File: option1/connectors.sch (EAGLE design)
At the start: 14 parts, among them CON1 PINHEAD_1X06-2, CON2 PINHEAD_1X03-2.54-RA, CON3 CON-4P-JST_GH-RA, CON4 PINHEAD_1X02-2, CON5 PINHEAD_1X02-2, CON8 CON-4P-JST_GH-RA, IC3 TJA1051

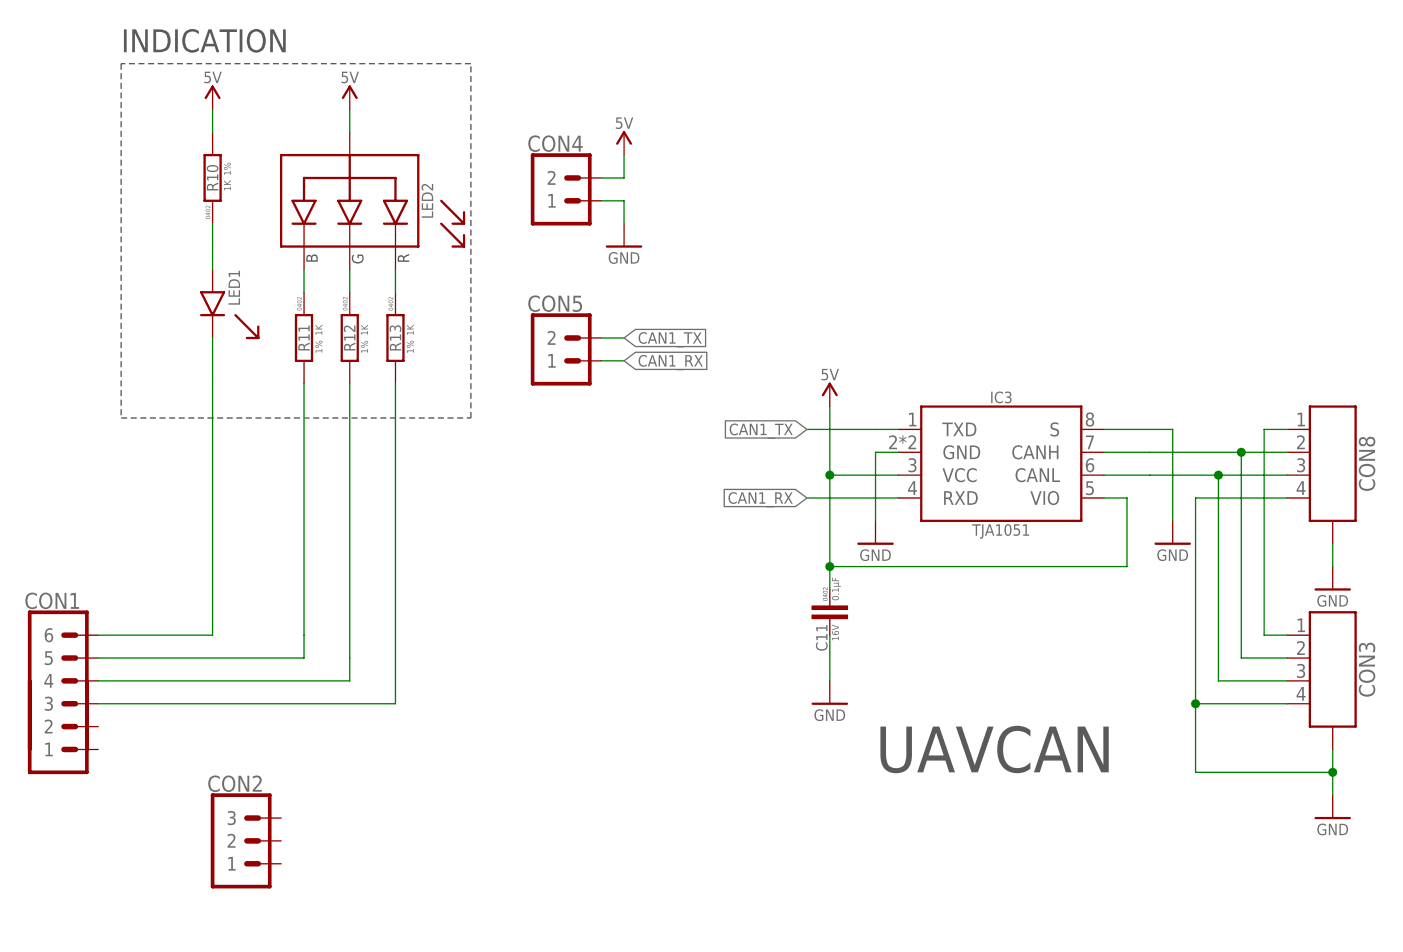
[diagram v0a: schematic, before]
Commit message: Roting is completed
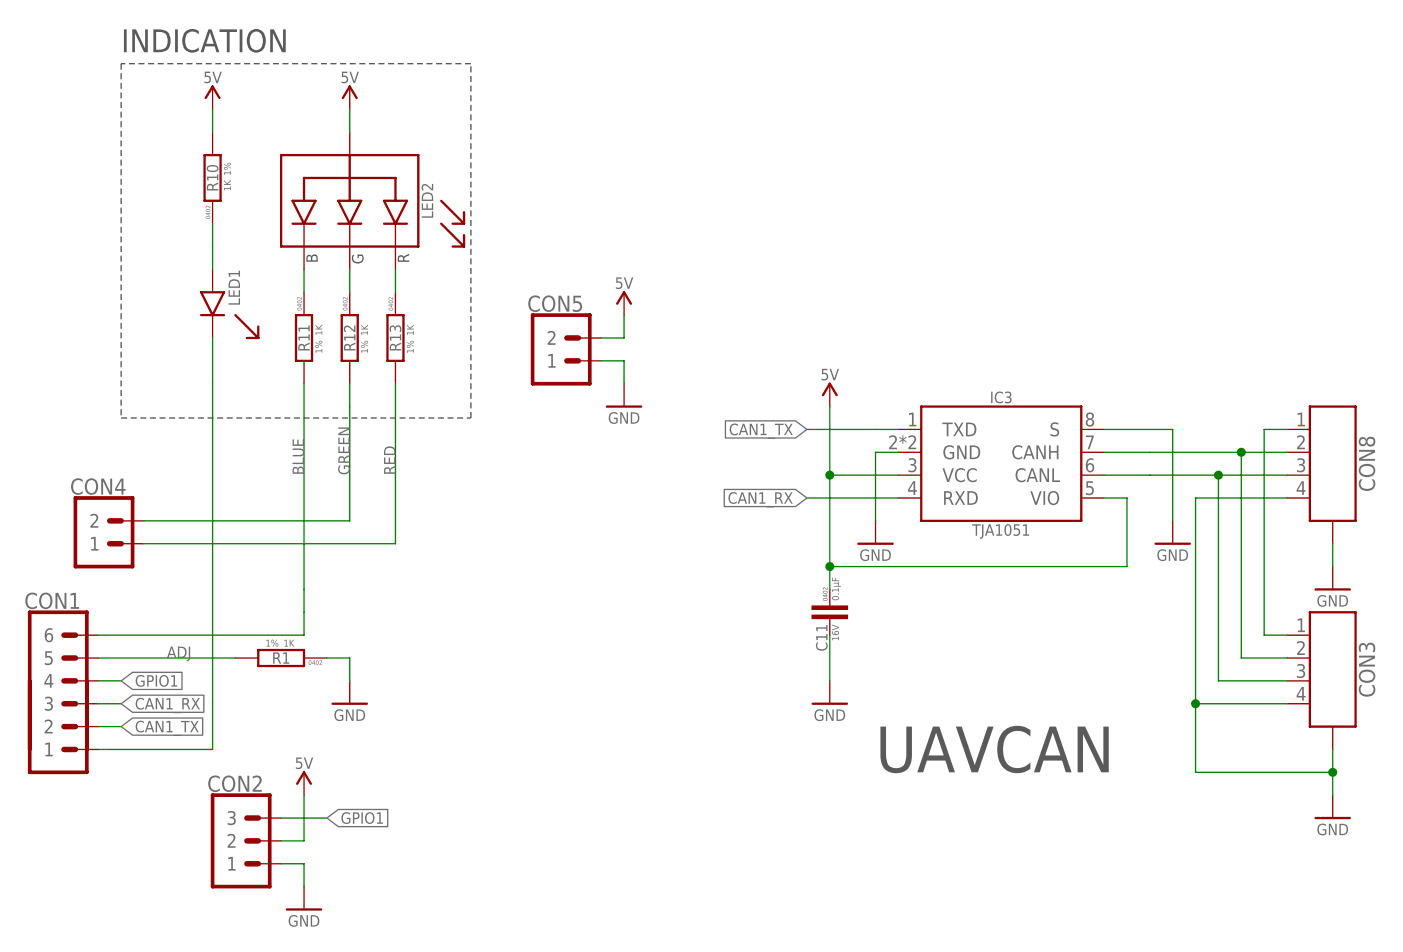
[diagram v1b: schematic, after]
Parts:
- added R1: 1K, R_digikey:1K-1%-0402
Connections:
- removed net LED_GREEN: CON1.4, R12.2
- removed net LED_RED: CON1.3, R13.2
- removed net N$6: CON1.5, R11.2
- new net ADJ: CON1.5, R1.2
- new net BLUE: CON1.6, R11.2
- new net GPIO1: CON1.4, CON2.3
- new net GREEN: CON4.2, R12.2
- new net RED: CON4.1, R13.2
- net CAN1_LED: now also CON1.1; no longer CON1.6
- net CAN1_RX: now also CON1.3; no longer CON5.1
- net CAN1_TX: now also CON1.2; no longer CON5.2
- net GND: now also CON2.1, CON5.1, R1.1; no longer CON4.1
- net VDD_5V: now also CON2.2, CON5.2; no longer CON4.2
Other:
- moved on the sheet: CON4
